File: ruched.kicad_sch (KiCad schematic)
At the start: 33 parts, among them J20 USB_C_Receptacle_USB2.0 USB41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, J23 USB_C_Receptacle_USB2.0 USB41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, Q6 UMH3N, Q7 DMG2301L, SW1 SW_Push, SW2 SW_Push, U1 CP2102N-A02-GQFN24, U8 ESP32-S3-WROOM-2

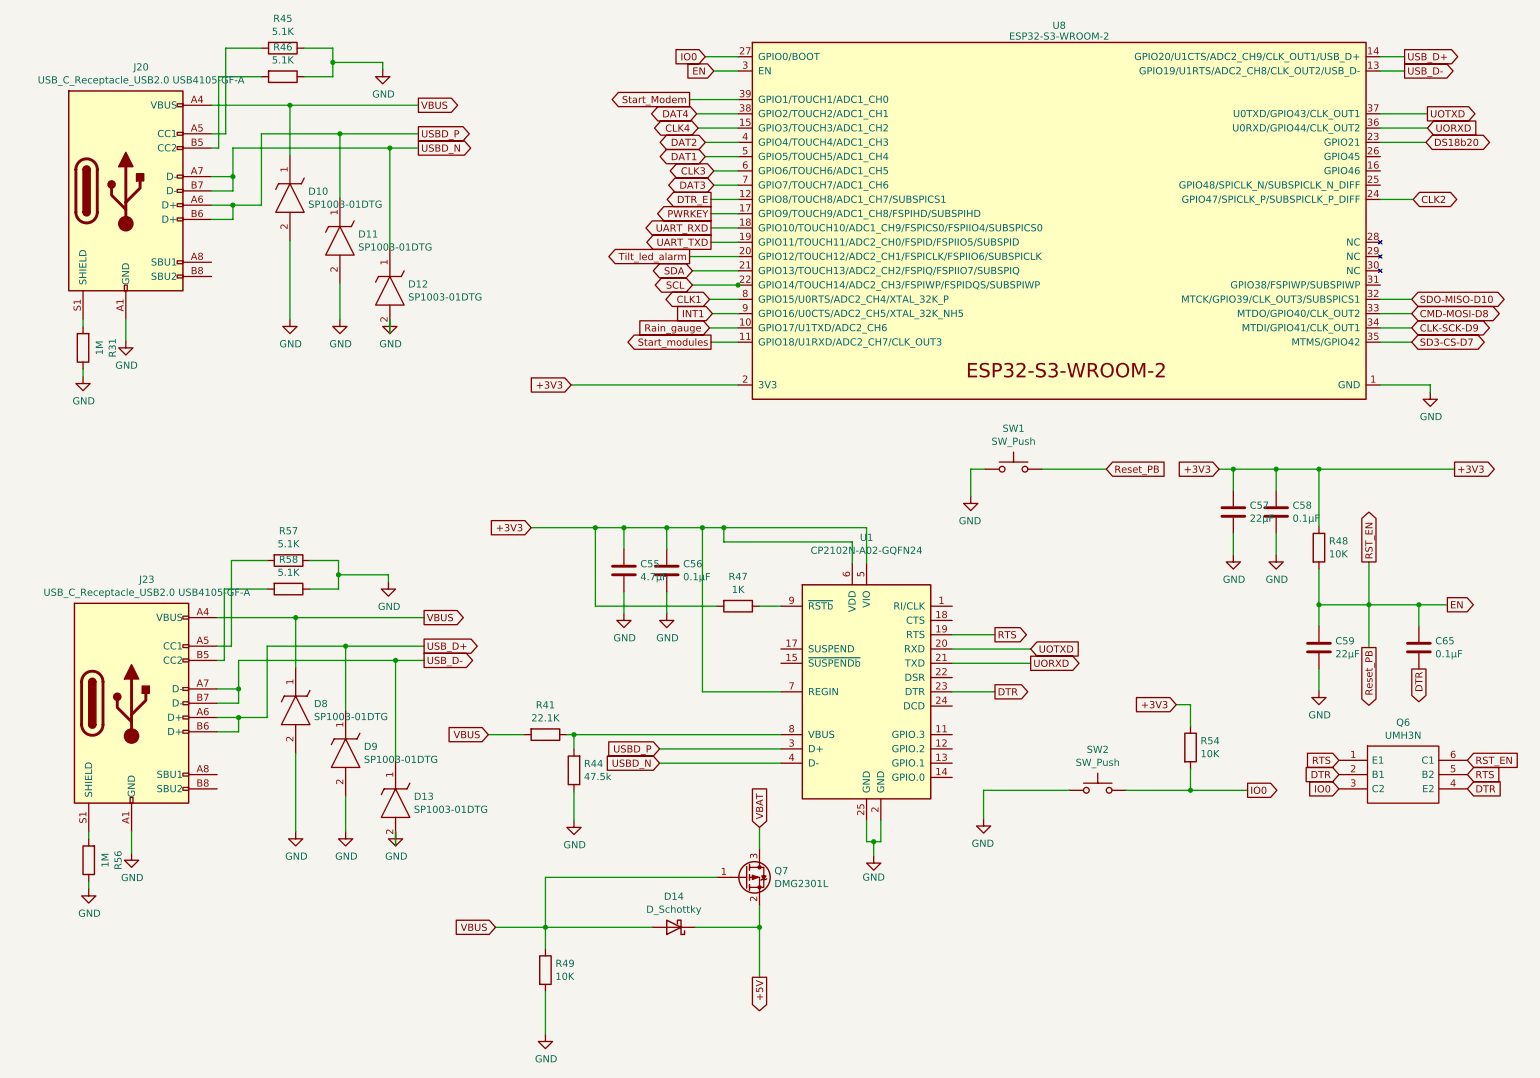
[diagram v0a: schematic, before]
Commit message: update
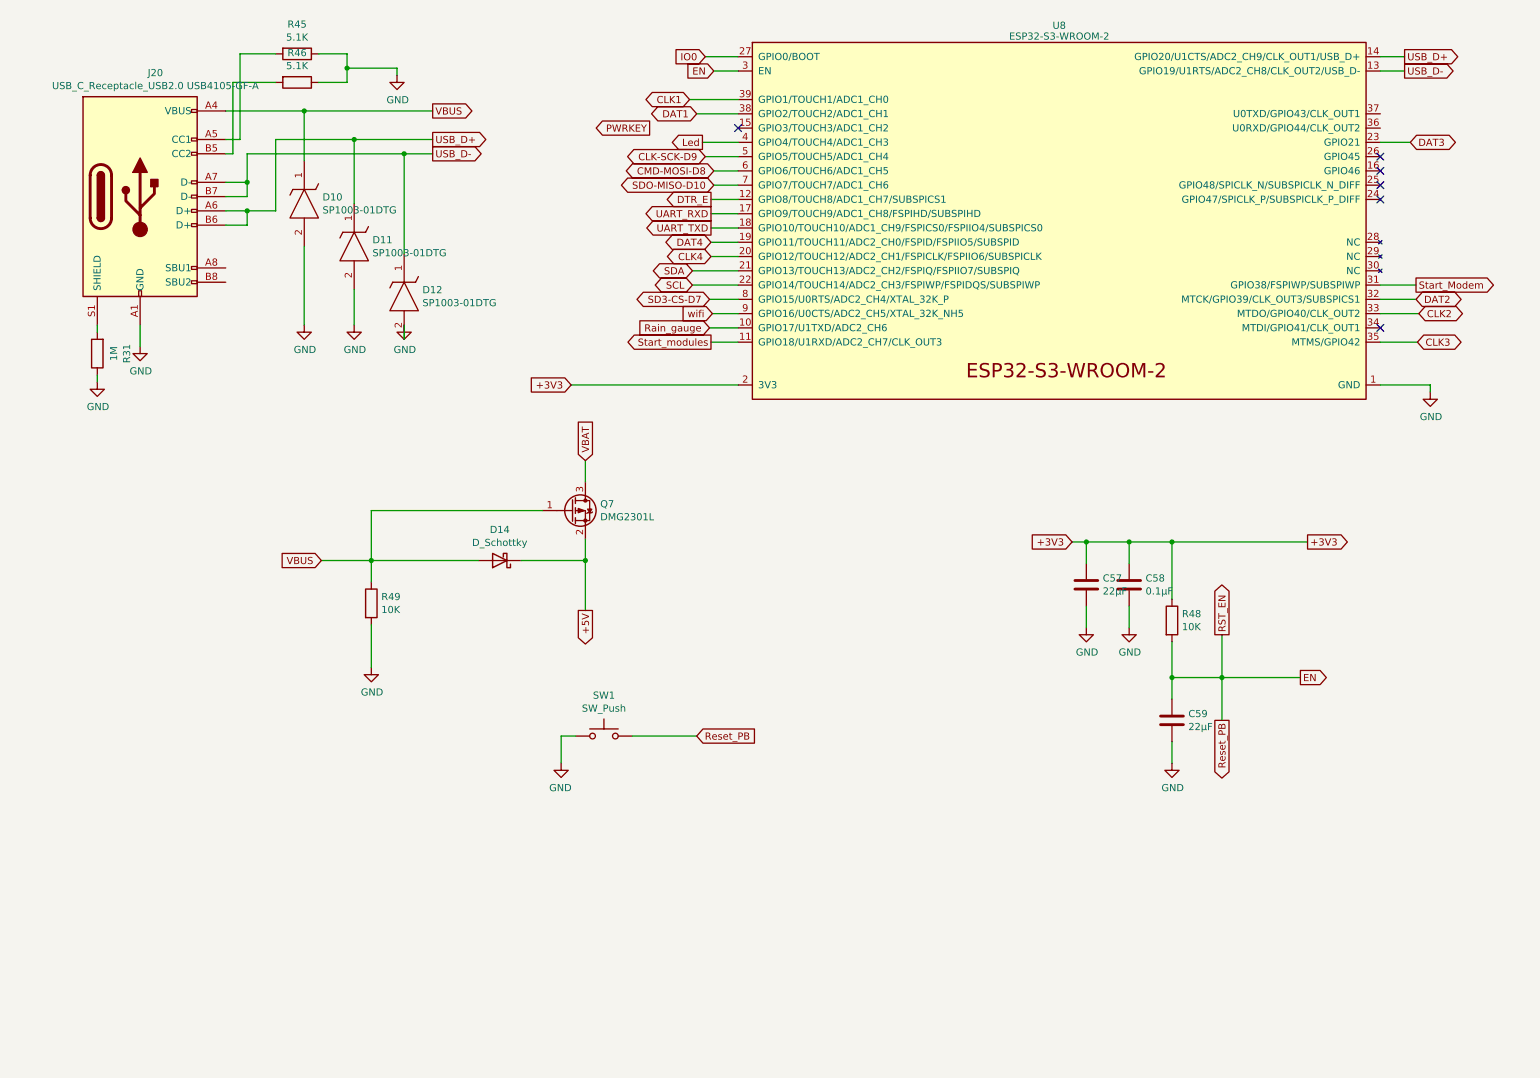
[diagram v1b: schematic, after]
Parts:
- removed C55: 4.7µF, Capacitor_SMD:C_0805_2012Metric, symbol Device:C
- removed C56, C65: 0.1µF, Capacitor_SMD:C_0603_1608Metric, symbol Device:C
- removed D10, D11, D12: SP1003-01DTG, Empreintes:SODFL1406X65N, symbol SP1003-01DTG:SP1003-01DTG
- removed J20: USB_C_Receptacle_USB2.0 USB4105-GF-A, Empreintes:TYPE-C-31-M-12, symbol Connector:USB_C_Receptacle_USB2.0
- removed Q6: UMH3N, Package_TO_SOT_SMD:SOT-363_SC-70-6, symbol UMH3N:UMH3N
- removed R31: 1M, Resistor_SMD:R_0603_1608Metric, symbol Device:R
- removed R41: 22.1K, Resistor_SMD:R_0603_1608Metric, symbol Device:R
- removed R44: 47.5k, Resistor_SMD:R_0603_1608Metric, symbol Device:R
- removed R45, R46: 5.1K, Resistor_SMD:R_0603_1608Metric, symbol Device:R
- removed R47: 1K, Resistor_SMD:R_0603_1608Metric, symbol Device:R
- removed R54: 10K, Resistor_SMD:R_0603_1608Metric, symbol Device:R
- removed SW2: SW_Push, Empreintes:PTS636SL43SMTRLFS, symbol Switch:SW_Push
- removed U1: CP2102N-A02-GQFN24, Package_DFN_QFN:QFN-24-1EP_4x4mm_P0.5mm_EP2.6x2.6mm, symbol TestboardV2.3-rescue:CP2102N-A01-GQFN24-Interface_USB
- renumbered D8 to D10, D9 to D11, D13 to D12, J23 to J20, R56 to R31, R57 to R45, R58 to R46
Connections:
- net DS18b20 is gone; now on net DAT3: U8.23 (GPIO21)
- net Tilt_led_alarm is gone; now on net CLK4: U8.20 (GPIO12/TOUCH12/ADC2_CH1/FSPICLK/FSPIIO6/SUBSPICLK)
- net CLK-SCK-D9: now also U8.5 (GPIO5/TOUCH5/ADC1_CH4); no longer U8.34 (MTDI/GPIO41/CLK_OUT1)
- net CLK1: now also U8.39 (GPIO1/TOUCH1/ADC1_CH0); no longer U8.8 (GPIO15/U0RTS/ADC2_CH4/XTAL_32K_P)
- net CLK2: now also U8.33 (MTDO/GPIO40/CLK_OUT2); no longer U8.24 (GPIO47/SPICLK_P/SUBSPICLK_P_DIFF)
- net CLK3: now also U8.35 (MTMS/GPIO42); no longer U8.6 (GPIO6/TOUCH6/ADC1_CH5)
- net CLK4: no longer U8.15 (GPIO3/TOUCH3/ADC1_CH2)
- net CMD-MOSI-D8: now also U8.6 (GPIO6/TOUCH6/ADC1_CH5); no longer U8.33 (MTDO/GPIO40/CLK_OUT2)
- net DAT1: now also U8.38 (GPIO2/TOUCH2/ADC1_CH1); no longer U8.5 (GPIO5/TOUCH5/ADC1_CH4)
- net DAT2: now also U8.32 (MTCK/GPIO39/CLK_OUT3/SUBSPICS1); no longer U8.4 (GPIO4/TOUCH4/ADC1_CH3)
- net DAT3: no longer U8.7 (GPIO7/TOUCH7/ADC1_CH6)
- net DAT4: now also U8.19 (GPIO11/TOUCH11/ADC2_CH0/FSPID/FSPIIO5/SUBSPID); no longer U8.38 (GPIO2/TOUCH2/ADC1_CH1)
- net PWRKEY: no longer U8.17 (GPIO9/TOUCH9/ADC1_CH8/FSPIHD/SUBSPIHD)
- net SD3-CS-D7: now also U8.8 (GPIO15/U0RTS/ADC2_CH4/XTAL_32K_P); no longer U8.35 (MTMS/GPIO42)
- net SDO-MISO-D10: now also U8.7 (GPIO7/TOUCH7/ADC1_CH6); no longer U8.32 (MTCK/GPIO39/CLK_OUT3/SUBSPICS1)
- net Start_Modem: now also U8.31 (GPIO38/FSPIWP/SUBSPIWP); no longer U8.39 (GPIO1/TOUCH1/ADC1_CH0)
- net UART_RXD: now also U8.17 (GPIO9/TOUCH9/ADC1_CH8/FSPIHD/SUBSPIHD); no longer U8.18 (GPIO10/TOUCH10/ADC1_CH9/FSPICS0/FSPIIO4/SUBSPICS0)
- net UART_TXD: now also U8.18 (GPIO10/TOUCH10/ADC1_CH9/FSPICS0/FSPIIO4/SUBSPICS0); no longer U8.19 (GPIO11/TOUCH11/ADC2_CH0/FSPID/FSPIIO5/SUBSPID)
- net INT1 renamed wifi
- net UORXD: no longer names the net of U8.36 (U0RXD/GPIO44/CLK_OUT2)
- net UOTXD: no longer names the net of U8.37 (U0TXD/GPIO43/CLK_OUT1)
- new net Led: U8.4 (GPIO4/TOUCH4/ADC1_CH3)
- no-connect marks 0 -> 6
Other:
- moved on the sheet: C57, C58, C59, D10, D11, D12, D14, J20, Q7, R31, R45, R46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
